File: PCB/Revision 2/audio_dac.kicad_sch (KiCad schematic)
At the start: 10 parts, among them U9 WM8524CGEDT

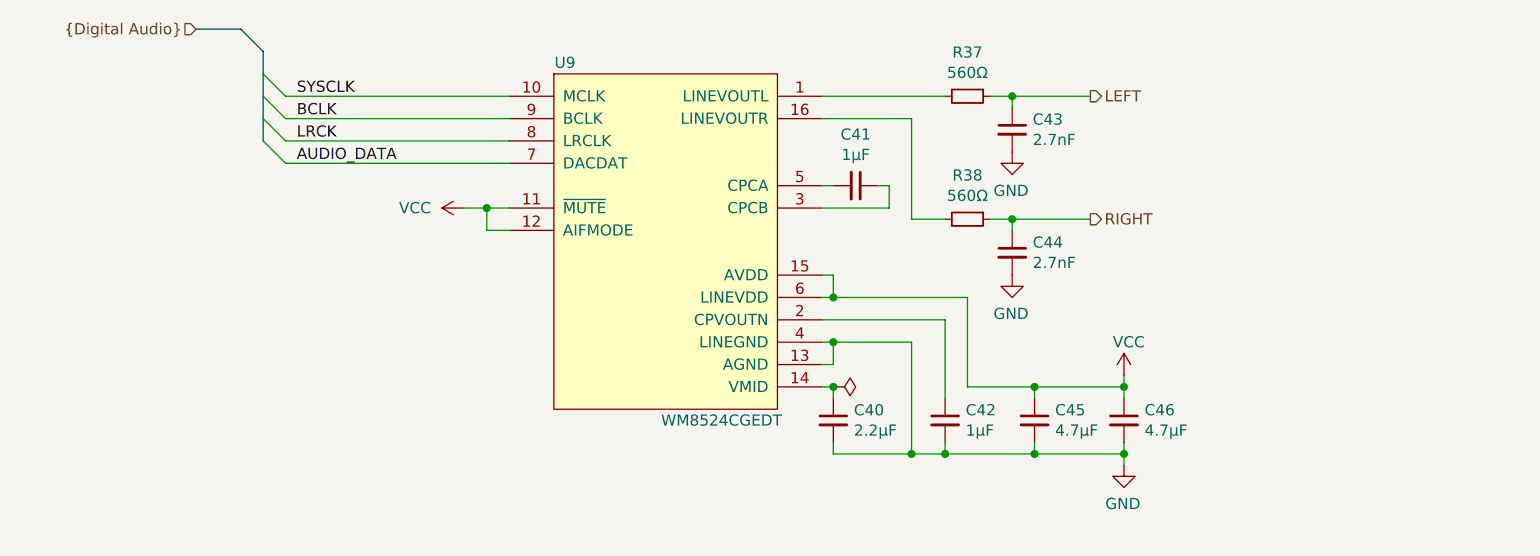
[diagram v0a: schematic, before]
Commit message: Updated re: issue #2
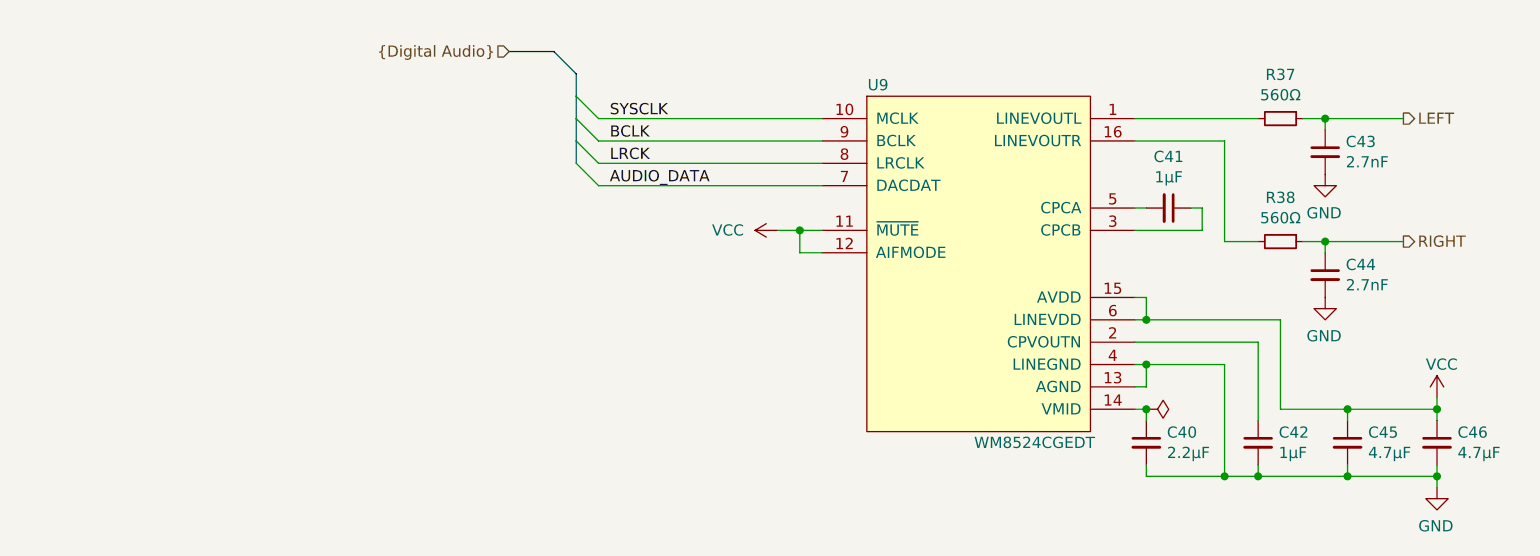
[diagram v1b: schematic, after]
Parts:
- C40, C41, C42, C43, C44, C45, C46: footprint (none) -> Capacitor_SMD:C_0402_1005Metric
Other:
- moved on the sheet: C40, C41, C42, C43, C44, C45, C46, R37, R38, U9
